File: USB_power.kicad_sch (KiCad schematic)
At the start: 24 parts, among them J4 TYPE-C-31-M12_13, J5 JST-4-pin, Q1 Q_NMOS, U3 TPD4E05U06DQAR, U4 BQ24074RGTR

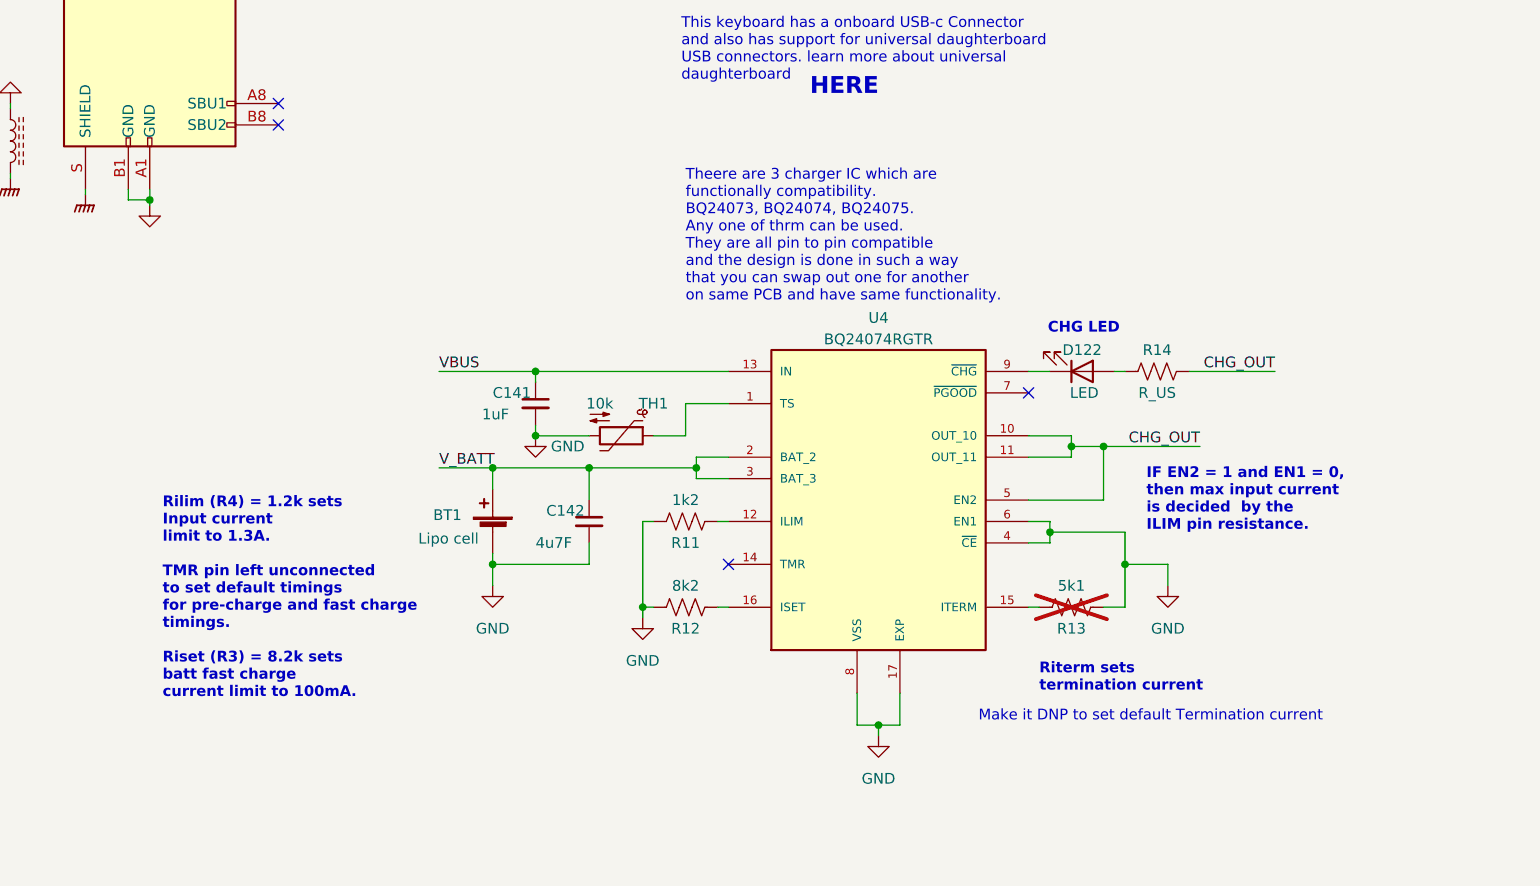
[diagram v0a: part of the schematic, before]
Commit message: Power supply and PCB stuff
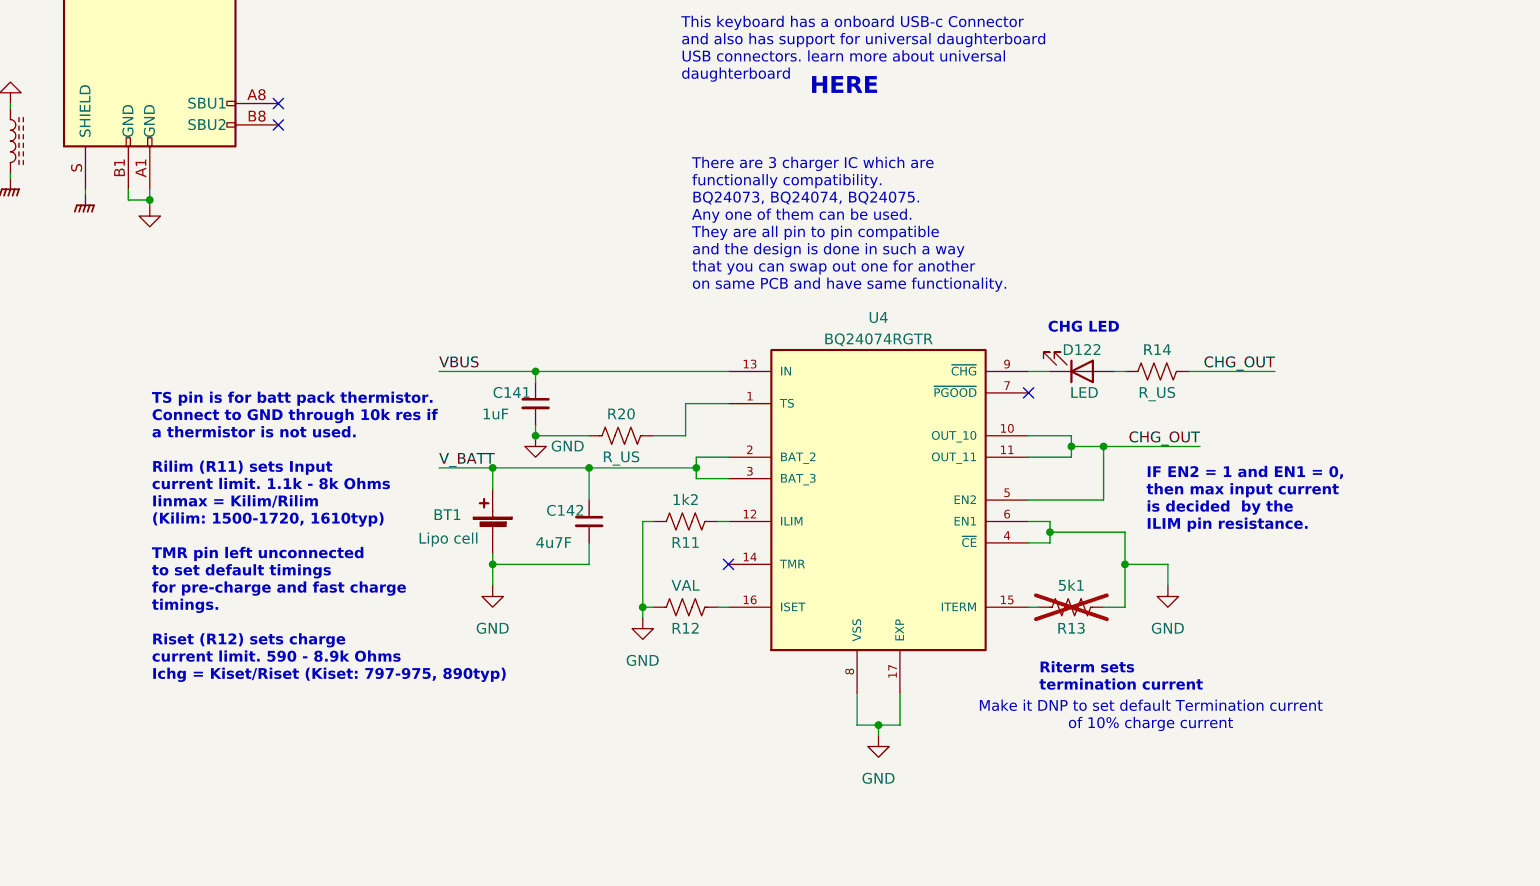
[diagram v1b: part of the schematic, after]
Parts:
- removed TH1: 10k, keyboard:R_0402_1005Metric, symbol keyboard:Thermistor_NTC
- added R20: R_US, keyboard:R_0402_1005Metric, symbol keyboard:R_US
- R12: value 8k2 -> VAL
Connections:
- net GND: now also R20.2
- net at U4.1 (TS): now also R20.1
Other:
- note added: "Make it DNP to set default Termination current of 10% charge current"
- note added: "TS pin is for batt pack thermistor. Connect to GND through 10k res if a thermistor is not used. Rilim (R11) sets Input current limit. 1.1k - 8k Ohms Iinmax = Kilim/Rilim (Kilim: 1500-1720, 1610typ) TMR pin left unconnected to set default timings for pre-charge and fast charge timings. Riset (R12) sets charge current limit. 590 - 8.9k Ohms Ichg = Kiset/Riset (Kiset: 797-975, 890typ)"
- note added: "There are 3 charger IC which are functionally compatibility. BQ24073, BQ24074, BQ24075. Any one of them can be used. They are all pin to pin compatible and the design is done in such a way that you can swap out one for another on same PCB and have same functionality."
- note removed: "Make it DNP to set default Termination current"
- note removed: "Rilim (R4) = 1.2k sets Input current limit to 1.3A. TMR pin left unconnected to set default timings for pre-charge and fast charge timings. Riset (R3) = 8.2k sets batt fast charge current limit to 100mA."
- note removed: "Theere are 3 charger IC which are functionally compatibility. BQ24073, BQ24074, BQ24075. Any one of thrm can be used. They are all pin to pin compatible and the design is done in such a way that you can swap out one for another on same PCB and have same functionality."
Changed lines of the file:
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@@
 		)
 	)
-	(text "Theere are 3 charger IC which are\nfunctionally compatibility.\nBQ24073, BQ24074, BQ24075.\nAny one of thrm can be used.\nThey are all pin to pin compatible \nand the design is done in such a way\nthat you can swap out one for another \non same PCB and have same functionality."
+	(text "There are 3 charger IC which are\nfunctionally compatibility.\nBQ24073, BQ24074, BQ24075.\nAny one of them can be used.\nThey are all pin to pin compatible \nand the design is done in such a way\nthat you can swap out one for another \non same PCB and have same functionality."
 		(exclude_from_sim no)
-		(at 113.03 103.632 0)
+		(at 113.792 102.362 0)
 		(effects
 			(font
@@
 		)
 	)
-	(text "Rilim (R4) = 1.2k sets \nInput current \nlimit to 1.3A.\n\nTMR pin left unconnected \nto set default timings \nfor pre-charge and fast charge\ntimings.\n\nRiset (R3) = 8.2k sets \nbatt fast charge \ncurrent limit to 100mA."
+	(text "TS pin is for batt pack thermistor.\nConnect to GND through 10k res if\na thermistor is not used.\n\nRilim (R11) sets Input\ncurrent limit. 1.1k - 8k Ohms\nIinmax = Kilim/Rilim\n(Kilim: 1500-1720, 1610typ)\n\nTMR pin left unconnected \nto set default timings \nfor pre-charge and fast charge\ntimings.\n\nRiset (R12) sets charge\ncurrent limit. 590 - 8.9k Ohms\nIchg = Kiset/Riset (Kiset: 797-975, 890typ)"
 		(exclude_from_sim no)
-		(at 51.054 150.622 0)
+		(at 49.784 148.59 0)
 		(effects
 			(font
@@
 		)
 	)
-	(text "Make it DNP to set default Termination current"
+	(text "Make it DNP to set default Termination current\nof 10% charge current"
 		(exclude_from_sim no)
 		(at 168.148 152.654 0)
@@
 	)
 	(symbol
-		(lib_id "keyboard:Thermistor_NTC")
-		(at 105.41 119.38 270)
-		(unit 1)
-		(exclude_from_sim no)
-		(in_bom yes)
-		(on_board yes)
-		(dnp no)
-		(property "Reference" "TH1"
-			(at 109.22 115.57 90)
-			(effects
-				(font
-					(size 1.27 1.27)
-				)
-			)
-		)
-		(property "Value" "10k"
-			(at 102.87 115.57 90)
-			(effects
-				(font
-					(size 1.27 1.27)
-				)
-			)
-		)
-		(property "Footprint" "keyboard:R_0402_1005Metric"
-			(at 106.68 119.38 0)
-			(effects
-				(font
-					(size 1.27 1.27)
-				)
-				(hide yes)
-			)
-		)
-		(property "Datasheet" "https://datasheet.lcsc.com/lcsc/2110081230_Sunlord-SDNT1005X103F3950FTF_C95939.pdf"
-			(at 106.68 119.38 0)
-			(effects
-				(font
-					(size 1.27 1.27)
-				)
-				(hide yes)
-			)
-		)
-		(property "Description" ""
-			(at 105.41 119.38 0)
-			(effects
-				(font
-					(size 1.27 1.27)
-				)
-				(hide yes)
-			)
-		)
-		(property "PN" "SDNT1005X103F3950FTF"
-			(at 105.41 119.38 0)
-			(effects
-				(font
-					(size 1.27 1.27)
-				)
-				(hide yes)
-			)
-		)
-		(property "LCSC Part Number" "C95939"
-			(at 105.41 119.38 0)
-			(effects
-				(font
-					(size 1.27 1.27)
-				)
-				(hide yes)
-			)
-		)
-		(property "LCSC link" "https://www.lcsc.com/product-detail/span-style-background-color-ff0-NTC-span-Thermistors_Sunlord-SDNT1005X103F3950FTF_C95939.html"
-			(at 105.41 119.38 0)
-			(effects
-				(font
-					(size 1.27 1.27)
-				)
-				(hide yes)
-			)
-		)
-		(pin "1"
-		)
-		(pin "2"
-		)
-		(instances
-			(project "Keyboard_60%"
-				(path "/ef112b03-6536-453f-8127-17d1495b48aa/01d5aa47-03a0-4747-998b-393b2b88e5ef"
-					(reference "TH1")
-					(unit 1)
-				)
-			)
-		)
-	)
-	(symbol
 		(lib_id "Unified-Daughterboard-rescue:TYPE-C-31-M12_13-acheronSymbols")
 		(at 49.53 53.34 0)
@@
 	)
 	(symbol
+		(lib_id "keyboard:R_US")
+		(at 105.41 119.38 0)
+		(unit 1)
+		(exclude_from_sim no)
+		(in_bom yes)
+		(on_board yes)
+		(dnp no)
+		(property "Reference" "R20"
+			(at 105.41 116.84 0)
+			(effects
+				(font
+					(size 1.27 1.27)
+				)
+			)
+		)
+		(property "Value" "R_US"
+			(at 105.41 121.92 0)
+			(effects
+				(font
+					(size 1.27 1.27)
+				)
+			)
+		)
+		(property "Footprint" "keyboard:R_0402_1005Metric"
+			(at 105.156 120.396 0)
+			(effects
+				(font
+					(size 1.27 1.27)
+				)
+				(hide yes)
+			)
+		)
+		(property "Datasheet" "https://datasheet.lcsc.com/lcsc/2304140030_YAGEO-RC0402FR-071K2L_C138040.pdf"
+			(at 105.41 119.38 90)
+			(effects
+				(font
+					(size 1.27 1.27)
+				)
+				(hide yes)
+			)
+		)
+		(property "Description" ""
+			(at 105.41 119.38 0)
+			(effects
+				(font
+					(size 1.27 1.27)
+				)
+				(hide yes)
+			)
+		)
+		(property "PN" "RC0402FR-071K2L"
+			(at 105.41 119.38 0)
+			(effects
+				(font
+					(size 1.27 1.27)
+				)
+				(hide yes)
+			)
+		)
+		(property "LCSC Part Number" "C138040"
+			(at 105.41 119.38 0)
+			(effects
+				(font
+					(size 1.27 1.27)
+				)
+				(hide yes)
+			)
+		)
+		(property "LCSC link" "https://www.lcsc.com/product-detail/Chip-Resistor-Surface-Mount_YAGEO-RC0402FR-071K2L_C138040.html"
+			(at 105.41 119.38 0)
+			(effects
+				(font
+					(size 1.27 1.27)
+				)
+				(hide yes)
+			)
+		)
+		(pin "1"
+		)
+		(pin "2"
+		)
+		(instances
+			(project "zmk-g915"
+				(path "/ef112b03-6536-453f-8127-17d1495b48aa/01d5aa47-03a0-4747-998b-393b2b88e5ef"
+					(reference "R20")
+					(unit 1)
+				)
+			)
+		)
+	)
+	(symbol
 		(lib_id "keyboard:JST-4-pin")
 		(at 135.89 59.69 0)
@@
 			)
 		)
-		(property "Value" "8k2"
+		(property "Value" "VAL"
 			(at 113.03 137.16 0)
 			(effects
